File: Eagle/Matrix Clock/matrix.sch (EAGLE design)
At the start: 63 parts, among them IC1 74HC595N, IC2 74HC595N, IC3 74HC595N, IC4 74HC595N, IC5 74HC595N

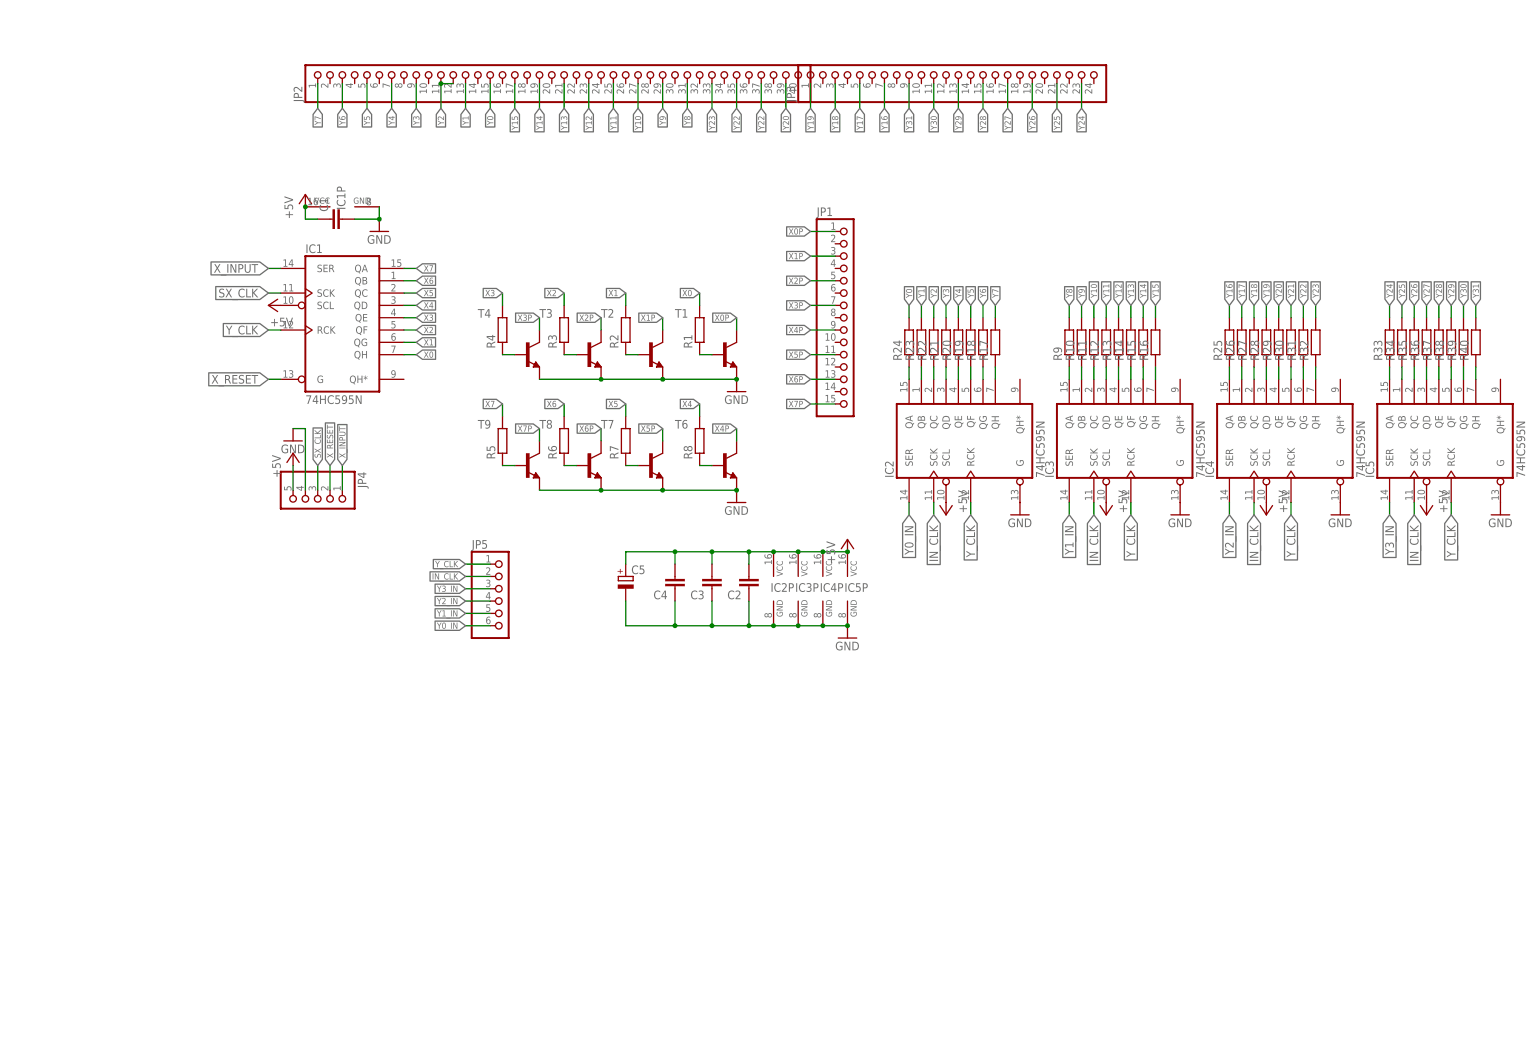
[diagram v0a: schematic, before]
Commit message: optymalizacja, UART
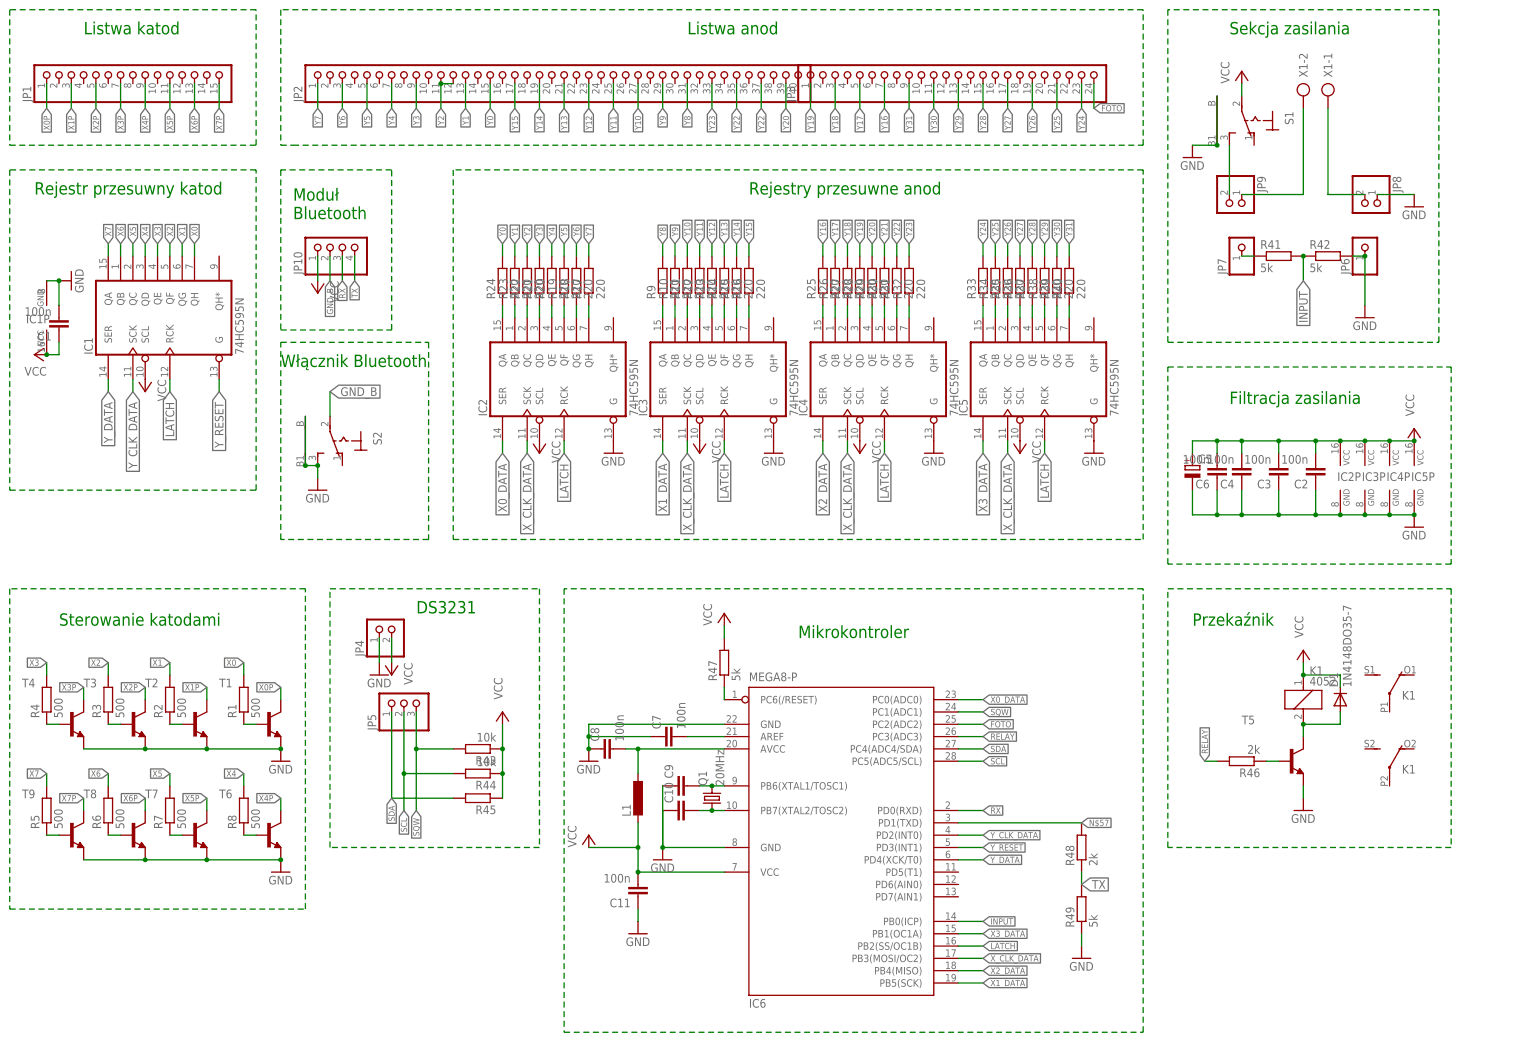
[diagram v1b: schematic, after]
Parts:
- added C10, C9: (no value), resistor:C-EU025-025X050
- added C11, C6, C7, C8: 100n, resistor:C-EU025-025X050
- added D1: 1N4148DO35-7, diode:1N4148DO35-7
- added IC6: MEGA8-P, atmel:MEGA8-P
- added JP10: (no value), pinhead:PINHD-1X4
- added JP6, JP7: (no value), pinhead:PINHD-1X1
- added JP8, JP9: (no value), pinhead:PINHD-1X2
- added K1: 4052, relay:4052
- added L1: (no value), resistor:L-EU0207/10
- added Q1: 20MHz, crystal:CRYSTALHC49S
- added R41, R42, R49: 5k, resistor:R-EU_0204/5
- added R43: 10k, resistor:R-EU_0207/7
- added R44: 10k, resistor:R-EU_0204/5
- added R45: (no value), resistor:R-EU_0204/5
- added R46: 2k, resistor:R-EU_0207/7
- added R47: 5k, resistor:R-EU_0204/2V
- added R48: 2k, resistor:R-EU_0204/5
- added S1, S2: (no value), switch:9070-1W
- added T5: (no value), transistor:BC337-16-NPN-TO92-CBE
- added X1: (no value), con-ptr500:AK300/2
- C1, C2, C3, C4: value (none) -> 100n; device resistor:C-EU050-025X075 -> resistor:C-EU025-025X050
- JP4: device pinhead:PINHD-1X5 -> pinhead:PINHD-1X2
- JP5: device pinhead:PINHD-1X6 -> pinhead:PINHD-1X3
- R1, R2, R3, R4, R5, R6, R7, R8: value (none) -> 500
- R10, R11, R12, R13, R14, R15, R16, R17, R20, R22, R23, R24, R25, R26, R27, R28, R29, R31, R32, R33, R34, R35, R37, R38, R39, R40, R9: value (none) -> 220
- R18, R19: value (none) -> 220; device resistor:R-EU_0204/5 -> resistor:R-EU_0204/2V
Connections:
- removed net IN_CLK: IC2A.SCK, IC3A.SCK, IC4A.SCK, IC5A.SCK, JP5.2
- removed net SX_CLK: IC1A.SCK, JP4.3
- removed net X_INPUT: IC1A.SER, JP4.1
- removed net X_RESET: IC1A.G, JP4.2
- removed net Y0_IN: IC2A.SER, JP5.6
- removed net Y1_IN: IC3A.SER, JP5.5
- removed net Y2_IN: IC4A.SER, JP5.4
- removed net Y3_IN: IC5A.SER, JP5.3
- removed net Y_CLK: IC1A.RCK, IC2A.RCK, IC3A.RCK, IC4A.RCK, IC5A.RCK, JP5.1
- new net FOTO: IC6.PC2(ADC2), JP3.24
- new net GND_B: JP10.2, S2.P
- new net INPUT: IC6.PB0(ICP), R41.2, R42.1
- new net LATCH: IC1A.RCK, IC2A.RCK, IC3A.RCK, IC4A.RCK, IC5A.RCK, IC6.PB2(SS/OC1B)
- new net N$11: JP8.2, X1-1.KL
- new net N$14: JP7.1, R41.1
- new net N$2: JP9.1, X1-2.KL
- new net N$36: JP9.2, S1.S
- new net N$41: C9.2, IC6.PB6(XTAL1/TOSC1), Q1.2
- new net N$42: C10.2, IC6.PB7(XTAL2/TOSC2), Q1.1
- new net N$43: C7.2, IC6.AREF
- new net N$52: C8.2, IC6.AVCC, L1.1
- new net N$53: D1.A, K11.2, T5.C
- new net N$54: R46.1, T5.B
- new net N$56: IC6.PC6(/RESET), R47.1
- new net N$57: IC6.PD1(TXD), R48.2
- new net RELAY: IC6.PC3(ADC3), R46.2
- new net RX: IC6.PD0(RXD), JP10.3
- new net SCL: IC6.PC5(ADC5/SCL), JP5.2, R44.2
- new net SDA: IC6.PC4(ADC4/SDA), JP5.1, R45.2
- new net SQW: IC6.PC1(ADC1), JP5.3, R43.2
- new net TX: JP10.4, R48.1, R49.2
- new net X0_DATA: IC2A.SER, IC6.PC0(ADC0)
- new net X1_DATA: IC3A.SER, IC6.PB5(SCK)
- new net X2_DATA: IC4A.SER, IC6.PB4(MISO)
- new net X3_DATA: IC5A.SER, IC6.PB1(OC1A)
- new net X_CLK_DATA: IC2A.SCK, IC3A.SCK, IC4A.SCK, IC5A.SCK, IC6.PB3(MOSI/OC2)
- new net Y_CLK_DATA: IC1A.SCK, IC6.PD2(INT0)
- new net Y_DATA: IC1A.SER, IC6.PD4(XCK/T0)
- new net Y_RESET: IC1A.G, IC6.PD3(INT1)
- net GND: now also C10.1, C11.1, C6.1, C7.1, C8.1, C9.1, IC6.GND, IC6.GND@1, JP4.1, JP6.1, JP8.1, R42.2, R49.1, S1.B, S1.B1, S2.B, S2.B1, S2.S, T5.E; no longer JP4.4
- net VCC: now also C11.2, C6.2, D1.C, IC6.VCC@1, JP10.1, JP4.2, K11.1, L1.2, R43.1, R44.1, R45.1, R47.2, S1.P; no longer JP4.5
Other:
- note added: "DS3231"
- note added: "Filtracja zasilania"
- note added: "Listwa anod"
- note added: "Listwa katod"
- note added: "Mikrokontroler"
- note added: "Moduł Bluetooth"
- note added: "Przekaźnik"
- note added: "Rejestr przesuwny katod"
- note added: "Rejestry przesuwne anod"
- note added: "Sekcja zasilania"
- note added: "Sterowanie katodami"
- note added: "Włącznik Bluetooth"
- moved on the sheet: C1, C2, C3, C4, C5, IC1, IC1P, IC2, IC2P, IC3, IC3P, IC4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
